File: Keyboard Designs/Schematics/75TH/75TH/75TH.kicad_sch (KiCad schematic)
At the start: 20 parts, among them J1 OLED_128x64, J2 USB_C_Receptacle_USB2.0_14P, SW1 RotaryEncoder_Switch_EC11E092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, U1 STM32F072CBTx

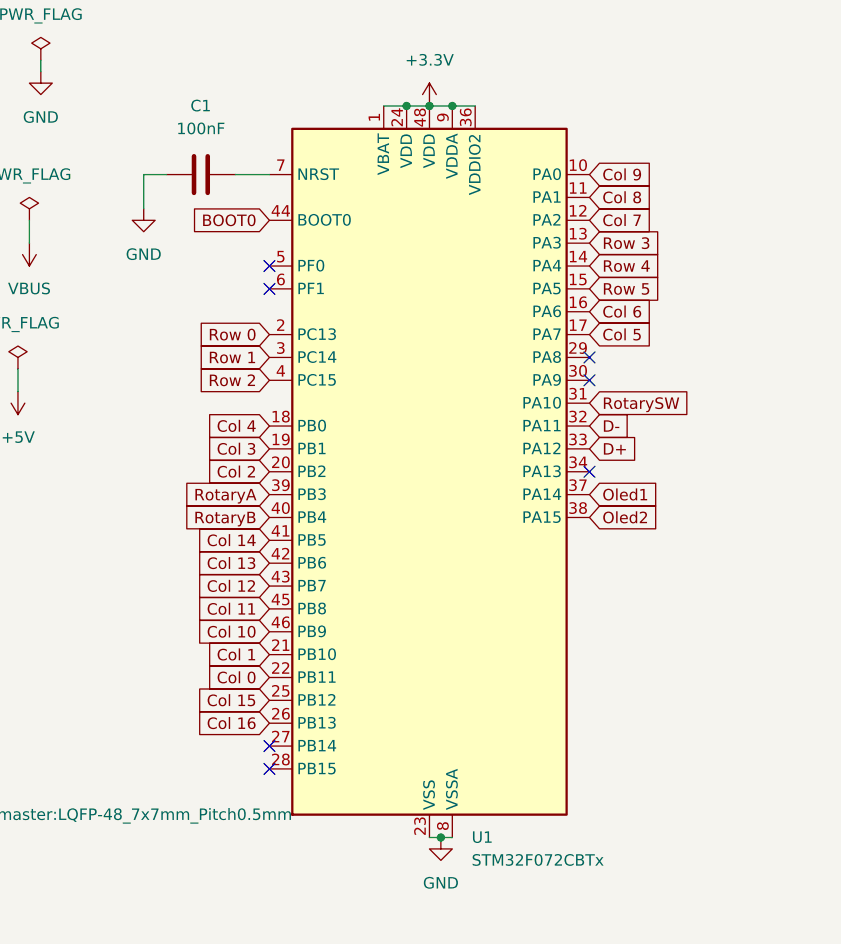
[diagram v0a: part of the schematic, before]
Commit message: Finished traces
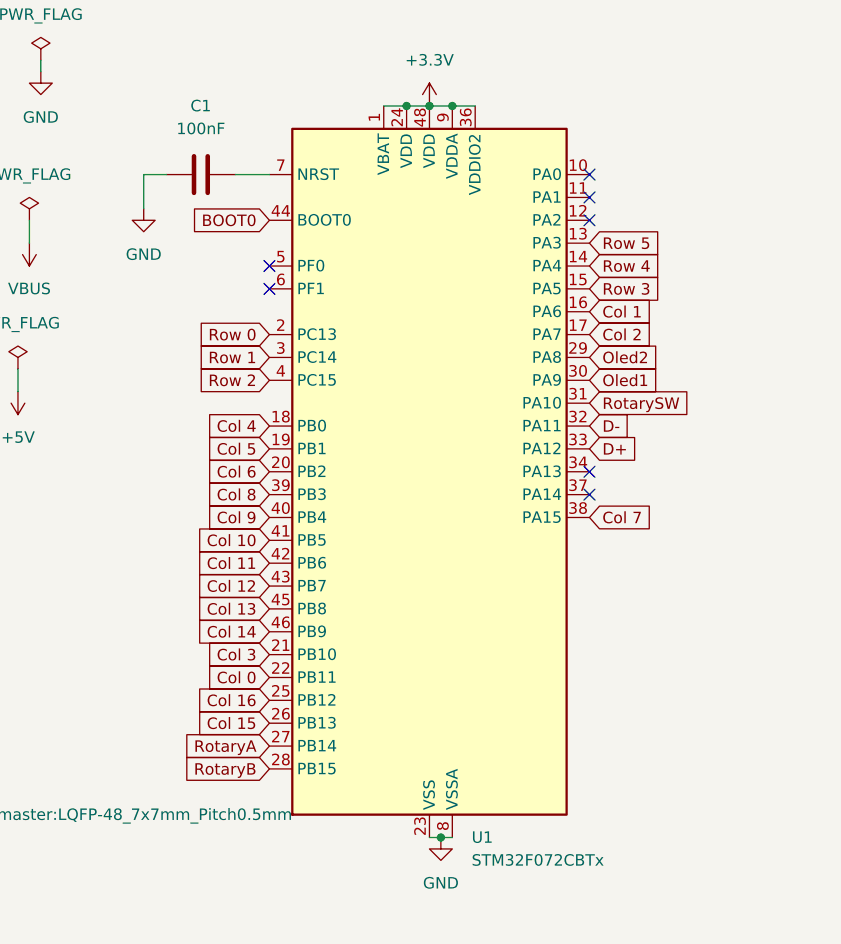
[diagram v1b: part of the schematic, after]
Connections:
- net Col 1: now also U1.16 (PA6); no longer U1.21 (PB10)
- net Col 10: now also U1.41 (PB5); no longer U1.46 (PB9)
- net Col 11: now also U1.42 (PB6); no longer U1.45 (PB8)
- net Col 13: now also U1.45 (PB8); no longer U1.42 (PB6)
- net Col 14: now also U1.46 (PB9); no longer U1.41 (PB5)
- net Col 15: now also U1.26 (PB13); no longer U1.25 (PB12)
- net Col 16: now also U1.25 (PB12); no longer U1.26 (PB13)
- net Col 2: now also U1.17 (PA7); no longer U1.20 (PB2)
- net Col 3: now also U1.21 (PB10); no longer U1.19 (PB1)
- net Col 5: now also U1.19 (PB1); no longer U1.17 (PA7)
- net Col 6: now also U1.20 (PB2); no longer U1.16 (PA6)
- net Col 7: now also U1.38 (PA15); no longer U1.12 (PA2)
- net Col 8: now also U1.39 (PB3); no longer U1.11 (PA1)
- net Col 9: now also U1.40 (PB4); no longer U1.10 (PA0)
- net Oled1: now also U1.30 (PA9); no longer U1.37 (PA14)
- net Oled2: now also U1.29 (PA8); no longer U1.38 (PA15)
- net RotaryA: now also U1.27 (PB14); no longer U1.39 (PB3)
- net RotaryB: now also U1.28 (PB15); no longer U1.40 (PB4)
- net Row 3: now also U1.15 (PA5); no longer U1.13 (PA3)
- net Row 5: now also U1.13 (PA3); no longer U1.15 (PA5)
